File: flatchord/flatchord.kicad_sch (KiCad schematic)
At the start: 9 parts, among them J1 OLED SSD1306, SW0 SW_SPST, SW1 SW_SPST, SW2 SW_SPST, SW3 SW_SPST, SW4 SW_SPST, SW5 SW_DPDT_x2, U2 Nice! Nano (ProMicro)

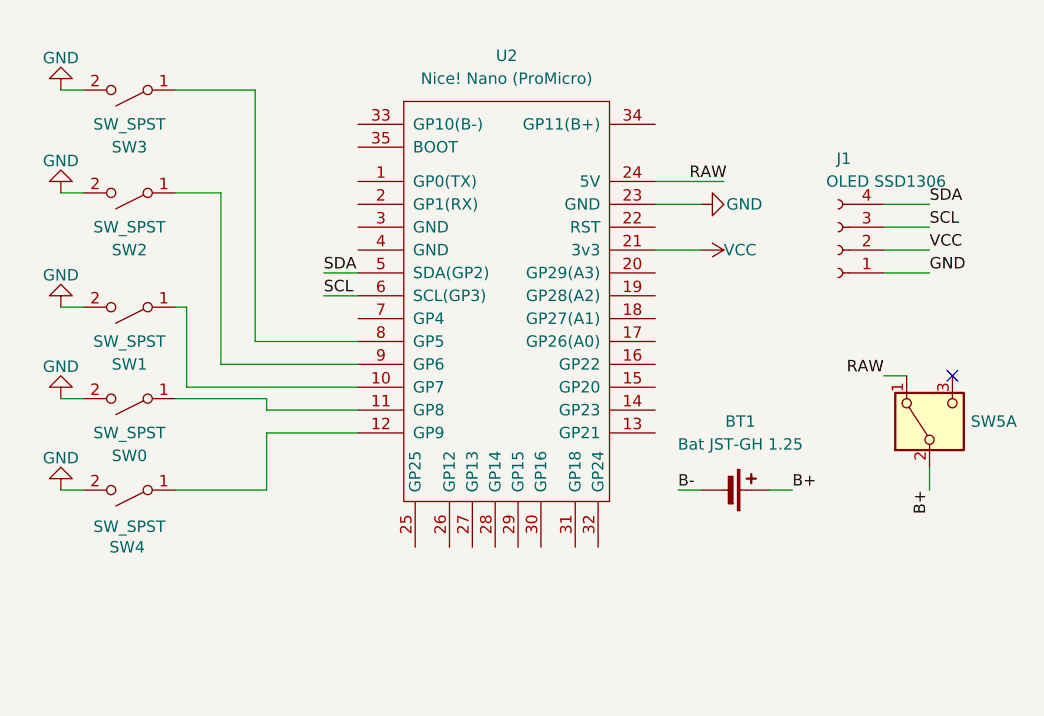
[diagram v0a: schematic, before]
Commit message: named board
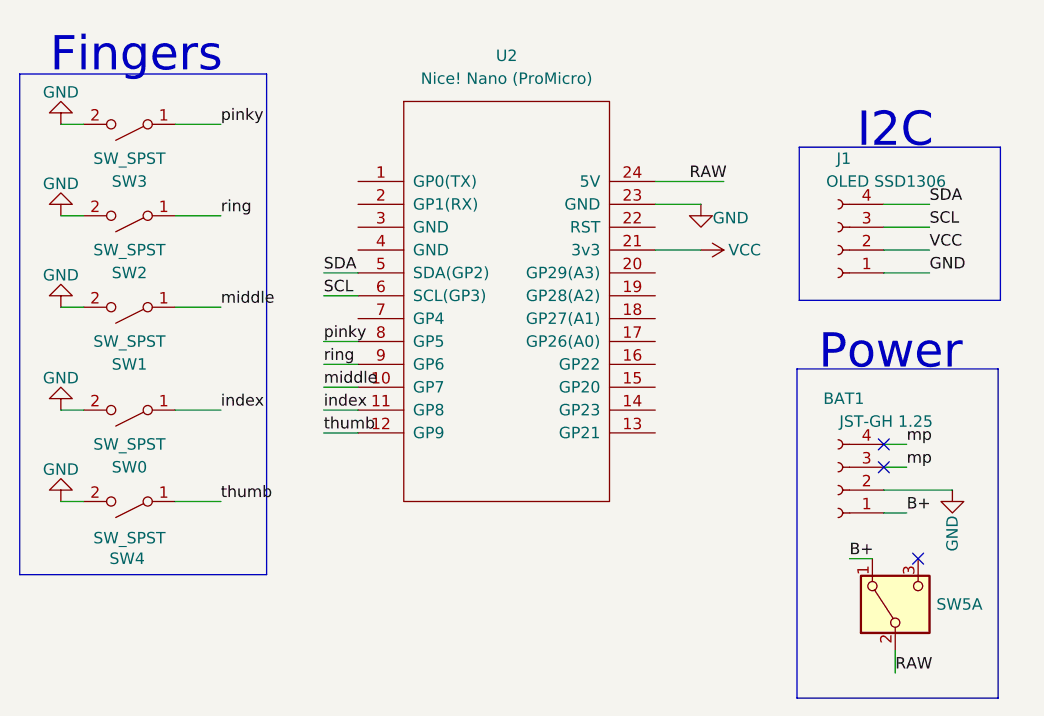
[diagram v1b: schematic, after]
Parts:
- removed BT1: Bat JST-GH 1.25, Connector_JST:JST_GH_SM02B-GHS-TB_1x02-1MP_P1.25mm_Horizontal, symbol Device:Battery_Cell
- added BAT1: JST-GH 1.25, footprints:JST_GH_SM02B-GHS-TB_1x02-1MP_P1.25mm_Horizontal, symbol Connector:Conn_01x04_Socket
- J1: footprint Connector_PinHeader_1.00mm:PinHeader_1x04_P1.00mm_Vertical_SMD_Pin1Right -> ssd1306-smd-header:lightblue-ssd1306-smd
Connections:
- net B+: now also SW5.1 (A), BAT1.1 (Pin_1); no longer SW5.2 (B)
- net GND: now also BAT1.2 (Pin_2)
- net RAW: now also SW5.2 (B); no longer SW5.1 (A)
- net middle: now reaches SW1.1 (A), U2.10 (GP7)
- net index: now reaches SW0.1 (A), U2.11 (GP8)
- net thumb: now reaches SW4.1 (A), U2.12 (GP9)
- net pinky: now reaches SW3.1 (A), U2.8 (GP5)
- net ring: now reaches SW2.1 (A), U2.9 (GP6)
- new net mp: BAT1.3 (Pin_3), BAT1.4 (Pin_4)
- no-connect marks 1 -> 3
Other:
- note added: "Fingers"
- note added: "I2C"
- note added: "Power"
- moved on the sheet: SW0, SW2, SW3, SW4, SW5A
